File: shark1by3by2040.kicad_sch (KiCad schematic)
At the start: 34 parts, among them SW1 BOOTSEL, SW2 Reset, U1 RP2040, U2 W25Q16JVSSIQ, U3 NCP1117-3.3_SOT223, Y1 ABLS-12.000MHZ-B4-T

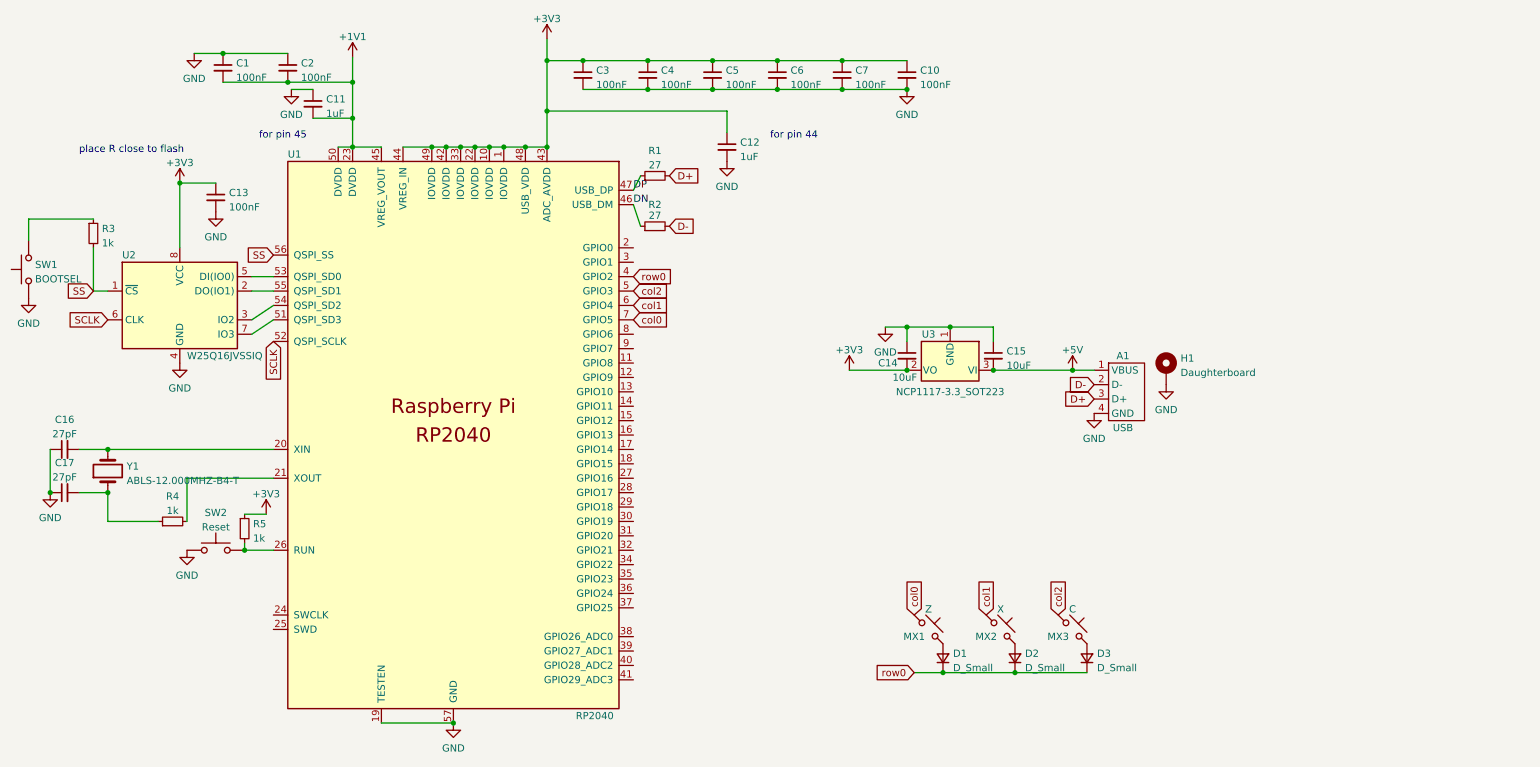
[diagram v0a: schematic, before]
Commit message: 1by3by2040 rev2
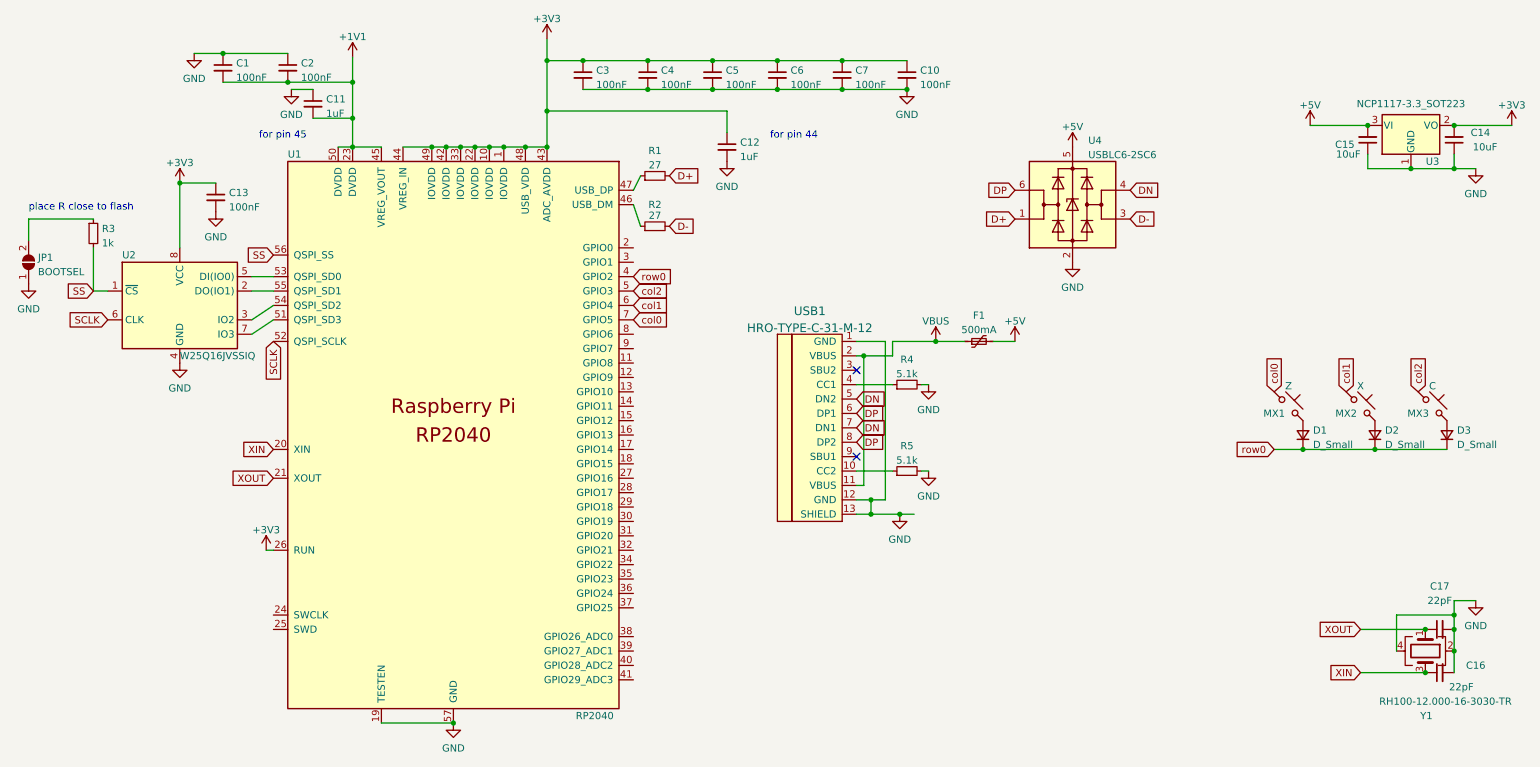
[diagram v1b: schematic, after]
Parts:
- removed A1: USB, random-keyboard-parts:JST-SR-4, symbol local:UNIFIED-DAUGHTERBOARD-C3
- removed H1: Daughterboard, local:UNIFIED-DAUGHTERBOARD-C3, symbol Mechanical:MountingHole_Pad
- removed SW1: BOOTSEL, local:TS-1187A, symbol Switch:SW_Push
- removed SW2: Reset, local:TS-1187A, symbol Switch:SW_Push
- added F1: 500mA, Fuse:Fuse_0805_2012Metric, symbol Device:Polyfuse_Small
- added JP1: BOOTSEL, random-keyboard-parts:Jumper-UserFriendly-Small, symbol Jumper:SolderJumper_2_Open
- added U4: USBLC6-2SC6, Package_TO_SOT_SMD:SOT-23-6, symbol Power_Protection:USBLC6-2SC6
- added USB1: HRO-TYPE-C-31-M-12, Type-C:HRO-TYPE-C-31-M-12-Assembly, symbol Type-C:HRO-TYPE-C-31-M-12
- C1, C10, C11, C12, C13, C14, C15, C2, C3, C4, C5, C6, C7: footprint Capacitor_SMD:C_0805_2012Metric -> Capacitor_SMD:C_0402_1005Metric
- C16, C17: value 27pF -> 22pF; footprint Capacitor_SMD:C_0805_2012Metric -> Capacitor_SMD:C_0402_1005Metric
- D1, D2, D3: footprint Diode_SMD:D_SOD-123 -> random-keyboard-parts:D_SOD-123-Pretty
- R1, R2, R3: footprint Resistor_SMD:R_0805_2012Metric -> Resistor_SMD:R_0402_1005Metric
- R4, R5: value 1k -> 5.1k; footprint Resistor_SMD:R_0805_2012Metric -> Resistor_SMD:R_0402_1005Metric
- Y1: value ABLS-12.000MHZ-B4-T -> RH100-12.000-16-3030-TR; footprint Crystal:Crystal_SMD_HC49-SD -> Crystal:Crystal_SMD_3225-4Pin_3.2x2.5mm; symbol Device:Crystal -> Device:Crystal_GND24
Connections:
- net +3V3: now also U1.26 (RUN); no longer R5.1
- net +5V: now also F1.2, U4.5 (VBUS)
- net D+: now also U4.1 (I/O1)
- net D-: now also U4.3 (I/O2)
- net DN: now also U4.4 (I/O2), USB1.5 (DN2), USB1.7 (DN1); no longer R2.1, U1.46 (USB_DM)
- net DP: now also U4.6 (I/O1), USB1.6 (DP1), USB1.8 (DP2); no longer R1.1, U1.47 (USB_DP)
- net GND: now also C16.2, C17.2, R4.2, R5.2, Y1.2, Y1.4, JP1.1 (A), U4.2 (GND), USB1.1 (GND), USB1.12 (GND), USB1.13 (SHIELD); no longer C16.1, C17.1
- net XOUT: now reaches U1.21 (XOUT)
- net XOUT: now also C17.1, Y1.1; no longer R4.2
- net at R3.1: now also JP1.2 (B)
- new net: R2.1, U1.46 (USB_DM)
- new net: R1.1, U1.47 (USB_DP)
- new net: R5.1, USB1.10 (CC2)
- new net: R4.1, USB1.4 (CC1)
- new net VBUS: F1.1, USB1.11 (VBUS), USB1.2 (VBUS)
- new net XIN: C16.1, U1.20 (XIN), Y1.3
- no-connect marks 0 -> 2
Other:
- moved on the sheet: C14, C15, C16, C17, D1, D2, D3, MX1, MX2, MX3, U3
